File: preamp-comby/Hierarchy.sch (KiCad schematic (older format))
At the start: 0 parts

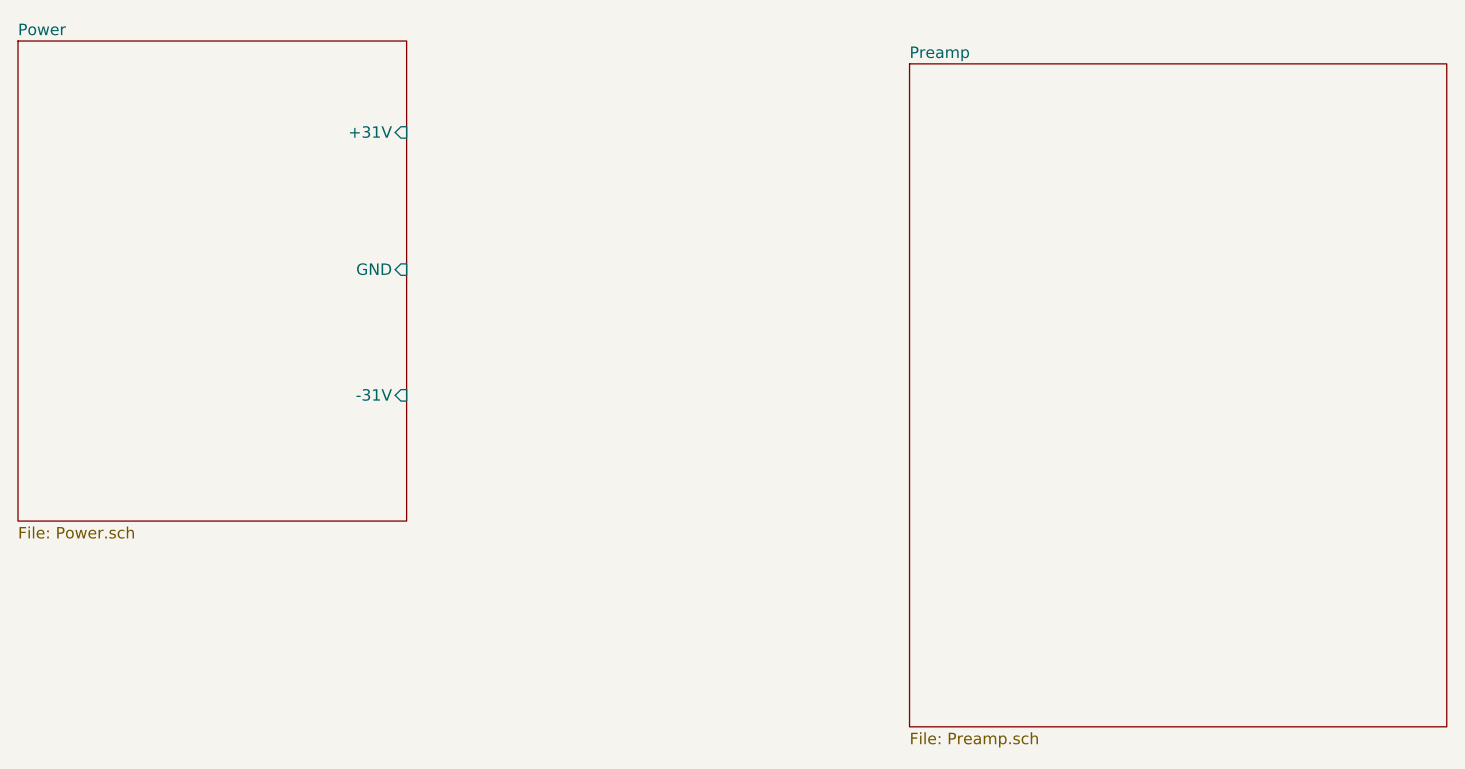
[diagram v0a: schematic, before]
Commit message: Finish schematic, start routing
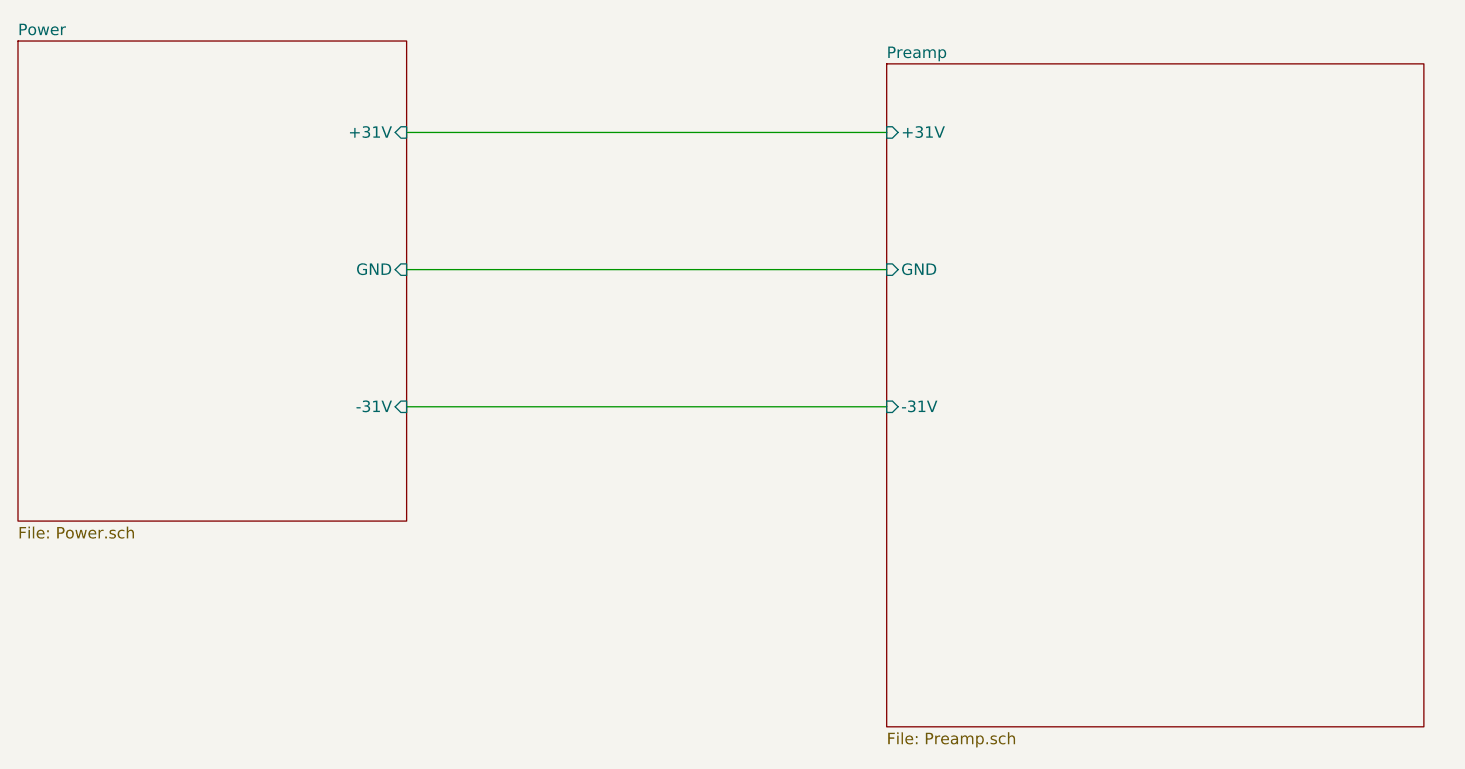
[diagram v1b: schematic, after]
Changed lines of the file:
@@
 EESchema Schematic File Version 4
+LIBS:Hierarchy-cache
 EELAYER 30 0
 EELAYER END
@@
 F0 "Power" 50
 F1 "Power.sch" 50
-F2 "-31V" I R 3850 3600 50
+F2 "-31V" I R 3850 3650 50
 F3 "+31V" I R 3850 2450 50
 F4 "GND" I R 3850 3050 50
 $EndSheet
 $Sheet
-S 6050 2150 2350 2900
+S 5950 2150 2350 2900
 U 5DA299FB
 F0 "Preamp" 50
 F1 "Preamp.sch" 50
+F2 "+31V" I L 5950 2450 50
+F3 "-31V" I L 5950 3650 50
+F4 "GND" I L 5950 3050 50
 $EndSheet
+Wire Wire Line
+	5950 3650 3850 3650
+Wire Wire Line
+	3850 3050 5950 3050
+Wire Wire Line
+	3850 2450 5950 2450
 $EndSCHEMATC
